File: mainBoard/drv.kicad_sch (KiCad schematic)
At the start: 9 parts, among them M1 Conn_01x01, M2 Conn_01x01, U2 DRV8251ADDAR

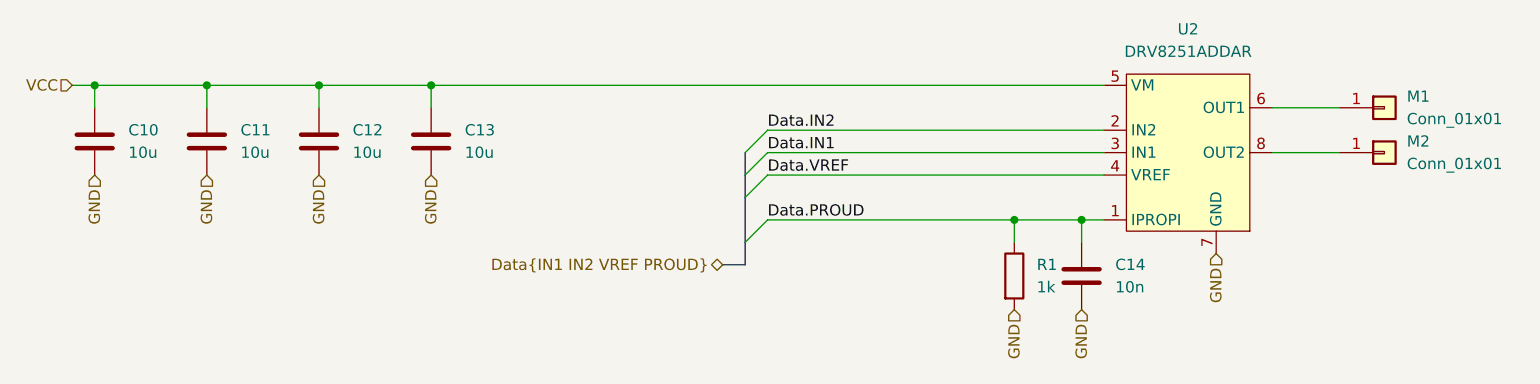
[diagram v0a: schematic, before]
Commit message: DebugBoard
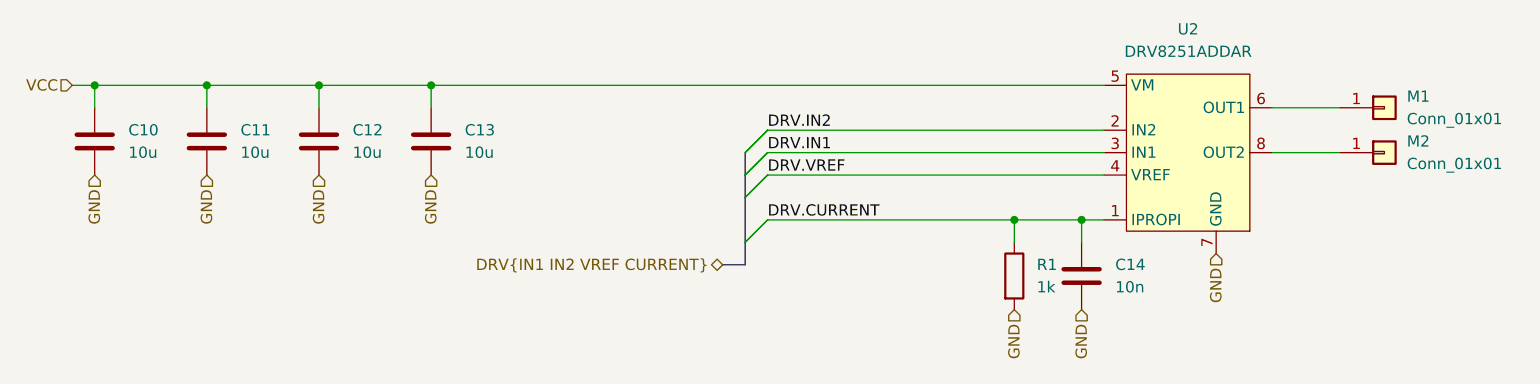
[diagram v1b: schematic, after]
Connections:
- net Data.IN1 renamed DRV.IN1
- net Data.IN2 renamed DRV.IN2
- net Data.PROUD renamed DRV.CURRENT
- net Data.VREF renamed DRV.VREF
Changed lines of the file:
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@@
   (junction (at 187.96 91.44) (diameter 0) (color 0 0 0 0)
+  )
+  (bus_entry (at 149.86 93.98) (size 2.54 -2.54)
+    (stroke (width 0) (type default))
   )
   (bus_entry (at 149.86 83.82) (size 2.54 -2.54)
     (stroke (width 0) (type default))
   )
+  (bus_entry (at 149.86 88.9) (size 2.54 -2.54)
+    (stroke (width 0) (type default))
+  )
   (bus_entry (at 149.86 86.36) (size 2.54 -2.54)
+    (stroke (width 0) (type default))
+  )
+  (bus_entry (at 149.86 83.82) (size 2.54 -2.54)
     (stroke (width 0) (type default))
   )
@@
   )
   (bus_entry (at 149.86 88.9) (size 2.54 -2.54)
+    (stroke (width 0) (type default))
+  )
+  (bus_entry (at 149.86 86.36) (size 2.54 -2.54)
     (stroke (width 0) (type default))
   )
@@
     (stroke (width 0) (type default))
   )
-  (label "Data.IN2" (at 152.4 81.28 0) (fields_autoplaced)
+  (label "DRV.CURRENT" (at 152.4 91.44 0)
     (effects (font (size 1.27 1.27)) (justify left bottom))
   )
-  (label "Data.VREF" (at 152.4 86.36 0) (fields_autoplaced)
+  (label "DRV.IN2" (at 152.4 81.28 0)
     (effects (font (size 1.27 1.27)) (justify left bottom))
   )
-  (label "Data.PROUD" (at 152.4 91.44 0) (fields_autoplaced)
+  (label "DRV.IN1" (at 152.4 83.82 0)
     (effects (font (size 1.27 1.27)) (justify left bottom))
   )
-  (label "Data.IN1" (at 152.4 83.82 0) (fields_autoplaced)
+  (label "DRV.VREF" (at 152.4 86.36 0)
     (effects (font (size 1.27 1.27)) (justify left bottom))
   )
@@
     (effects (font (size 1.27 1.27)) (justify right))
   )
-  (hierarchical_label "Data{IN1 IN2 VREF PROUD}" (shape bidirectional) (at 147.32 96.52 180) (fields_autoplaced)
+  (hierarchical_label "DRV{IN1 IN2 VREF CURRENT}" (shape bidirectional) (at 147.32 96.52 180) (fields_autoplaced)
     (effects (font (size 1.27 1.27)) (justify right))
   )
